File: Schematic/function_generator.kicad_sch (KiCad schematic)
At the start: 27 parts, among them J1 BNC, J2 Barrel_Jack, Q1 TIP41, Q2 TIP42, SW1 SW_SPDT, SW2 Top, SW3 Center, SW4 Bottom, U1 TL071, U2 AD9833, U3 STM32F103C8Tx, U4 LCD, U5 L7805, U6 LM358, U7 AMS1117-3.3

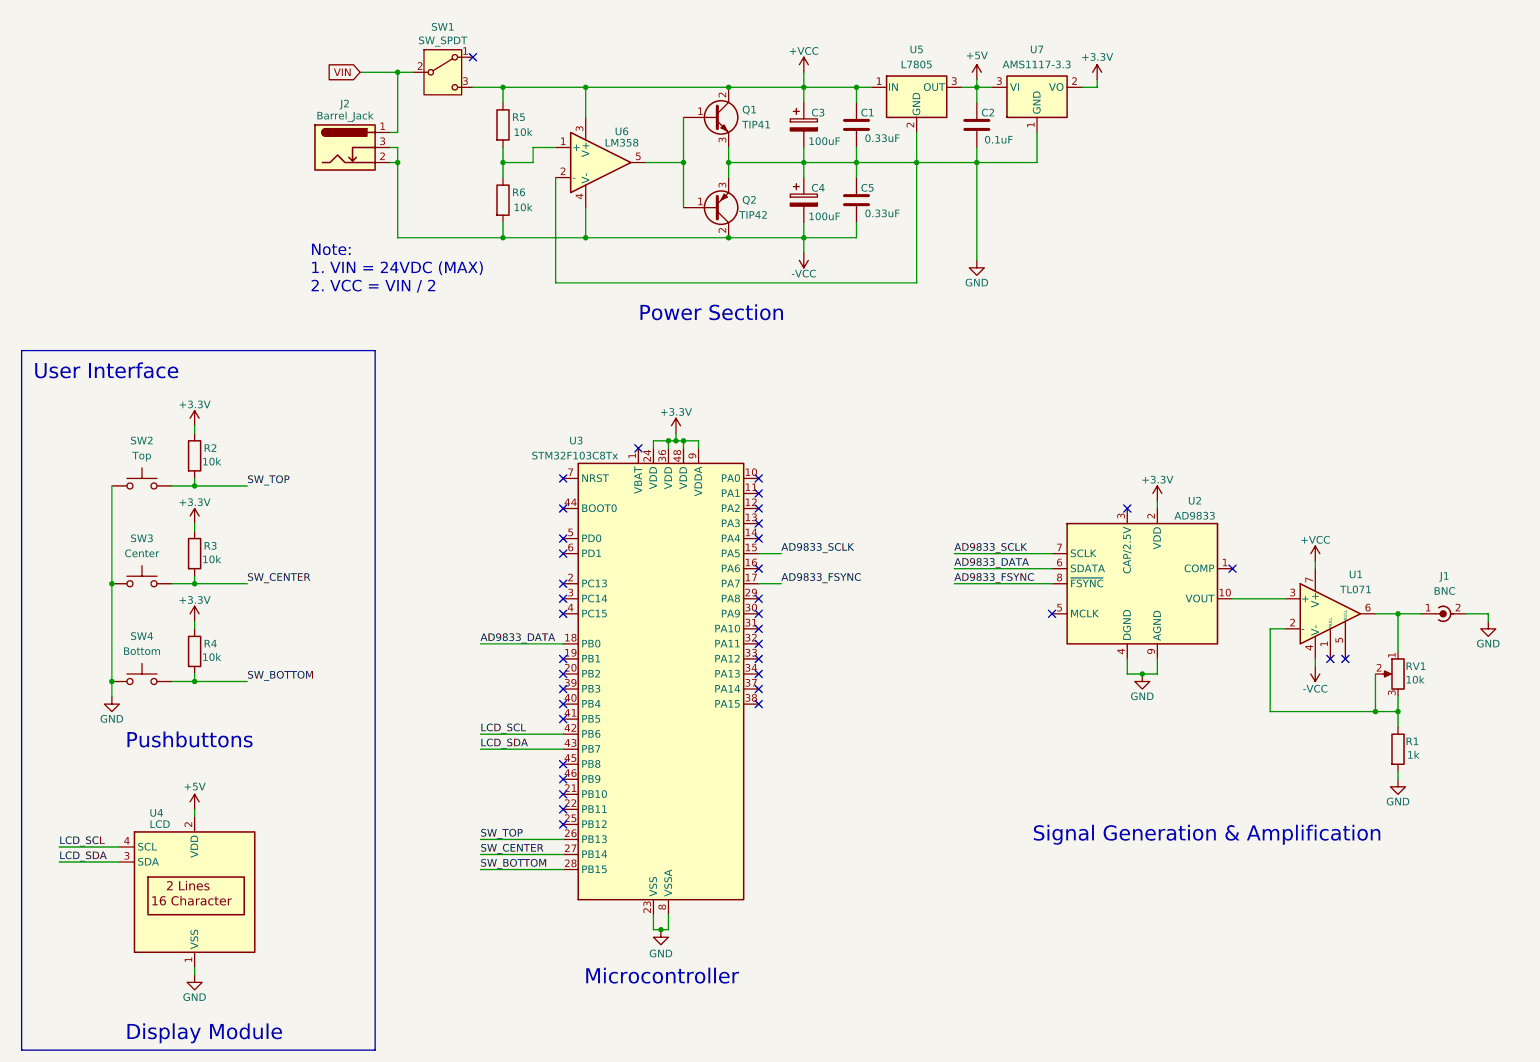
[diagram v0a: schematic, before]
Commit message: Update
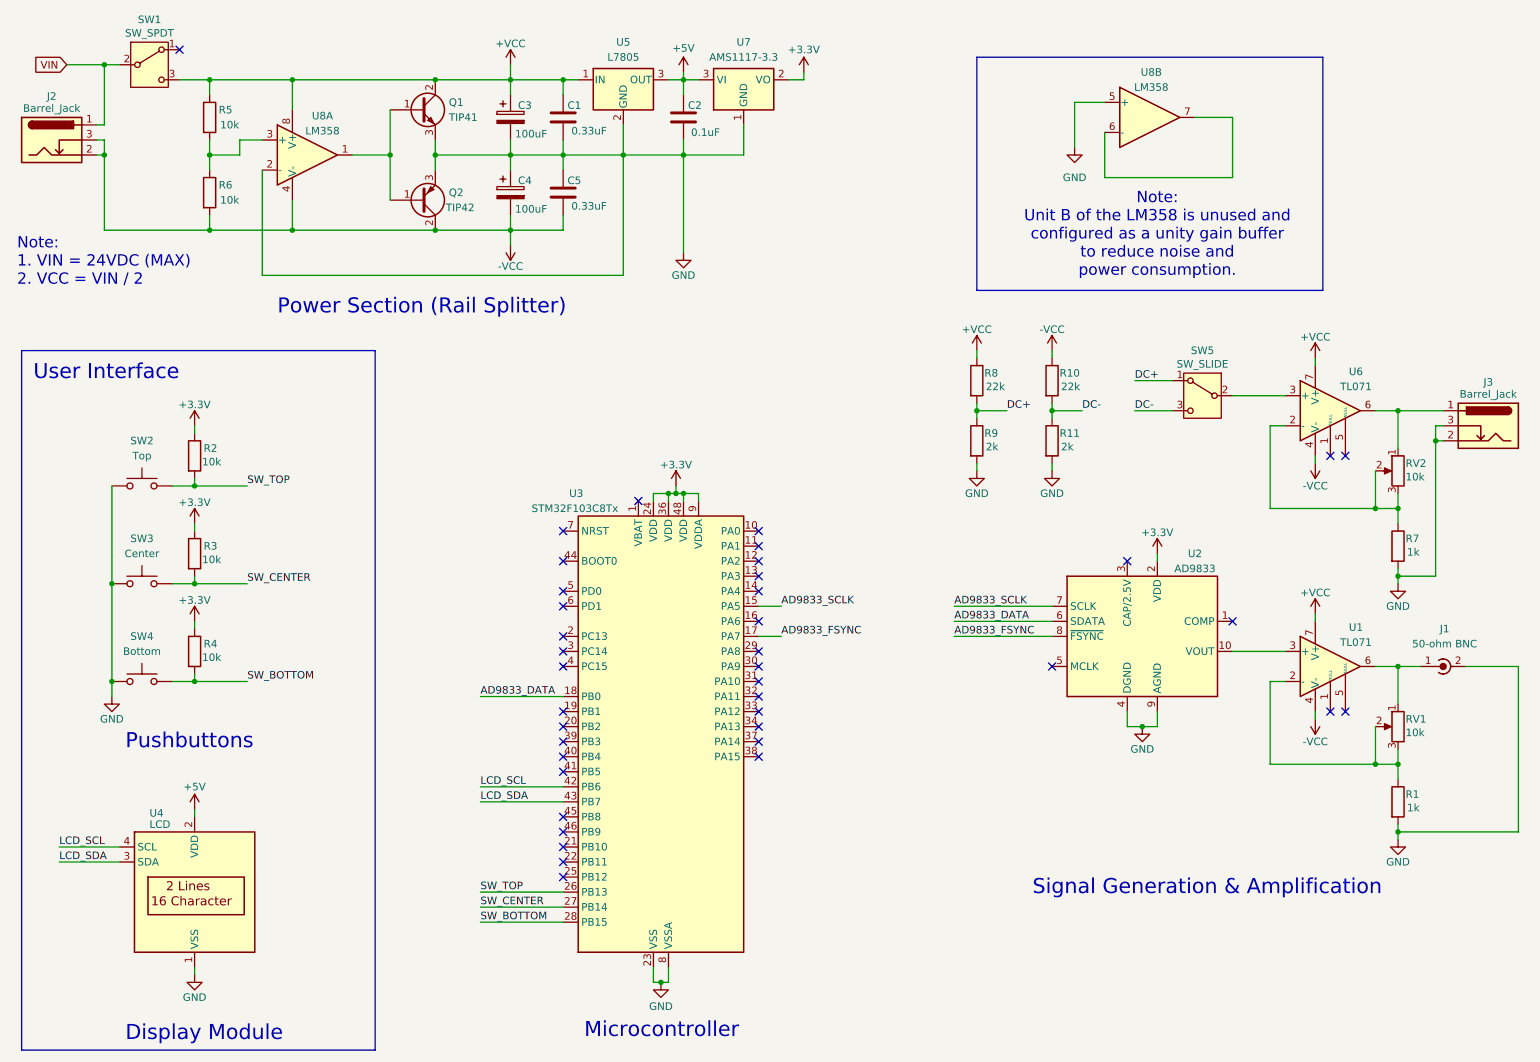
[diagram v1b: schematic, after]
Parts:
- removed U6: LM358, symbol Simulation_SPICE:OPAMP
- added J3: Barrel_Jack, symbol Connector:Barrel_Jack_Switch
- added R10, R8: 22k, symbol Device:R
- added R11, R9: 2k, symbol Device:R
- added R7: 1k, symbol Device:R
- added RV2: 10k, symbol Device:R_Potentiometer
- added SW5: SW_SLIDE, symbol Switch:SW_SPDT
- added U6: TL071, symbol Amplifier_Operational:TL071
- added U8: LM358, symbol Amplifier_Operational:LM358
- J1: value BNC -> 50-ohm BNC
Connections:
- net +VCC: now also R8.1, U6.7 (V+), U8.8 (V+)
- net -VCC: now also R10.1, U6.4 (V-), U8.4 (V-)
- net GND: now also J3.2, J3.3, R11.2, R7.2, R9.2, U8.2 (-), U8.5 (+)
- net at R5.2, R6.1: now also U8.3 (+)
- net at Q1.1 (B), Q2.1 (B): now also U8.1
- new net: U8.6 (-), U8.7
- new net: R7.1, RV2.2, RV2.3, U6.2 (-)
- new net: SW5.2 (B), U6.3 (+)
- new net: J3.1, RV2.1, U6.6
- new net DC+: R8.2, R9.1, SW5.1 (A)
- new net DC-: R10.2, R11.1, SW5.3 (C)
- no-connect marks 38 -> 40
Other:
- note added: "Note: Unit B of the LM358 is unused and configured as a unity gain buffer to reduce noise and power consumption."
- note added: "Power Section (Rail Splitter)"
- note removed: "Power Section"
- company: (none) -> Department of Electrical & Electronic Engineering, University of Ibadan
- title: (none) -> Custom Function Generator
- moved on the sheet: C1, C2, C3, C4, C5, J1, J2, Q1, Q2, R1, R5, R6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
